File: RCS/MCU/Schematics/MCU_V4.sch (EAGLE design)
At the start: 28 parts, among them IC1 FT232RL, J1 MOTOR, J2 POWER, J3 SENSORS, Q2 8 MHz, U1 ATMEGA328P_TQFP

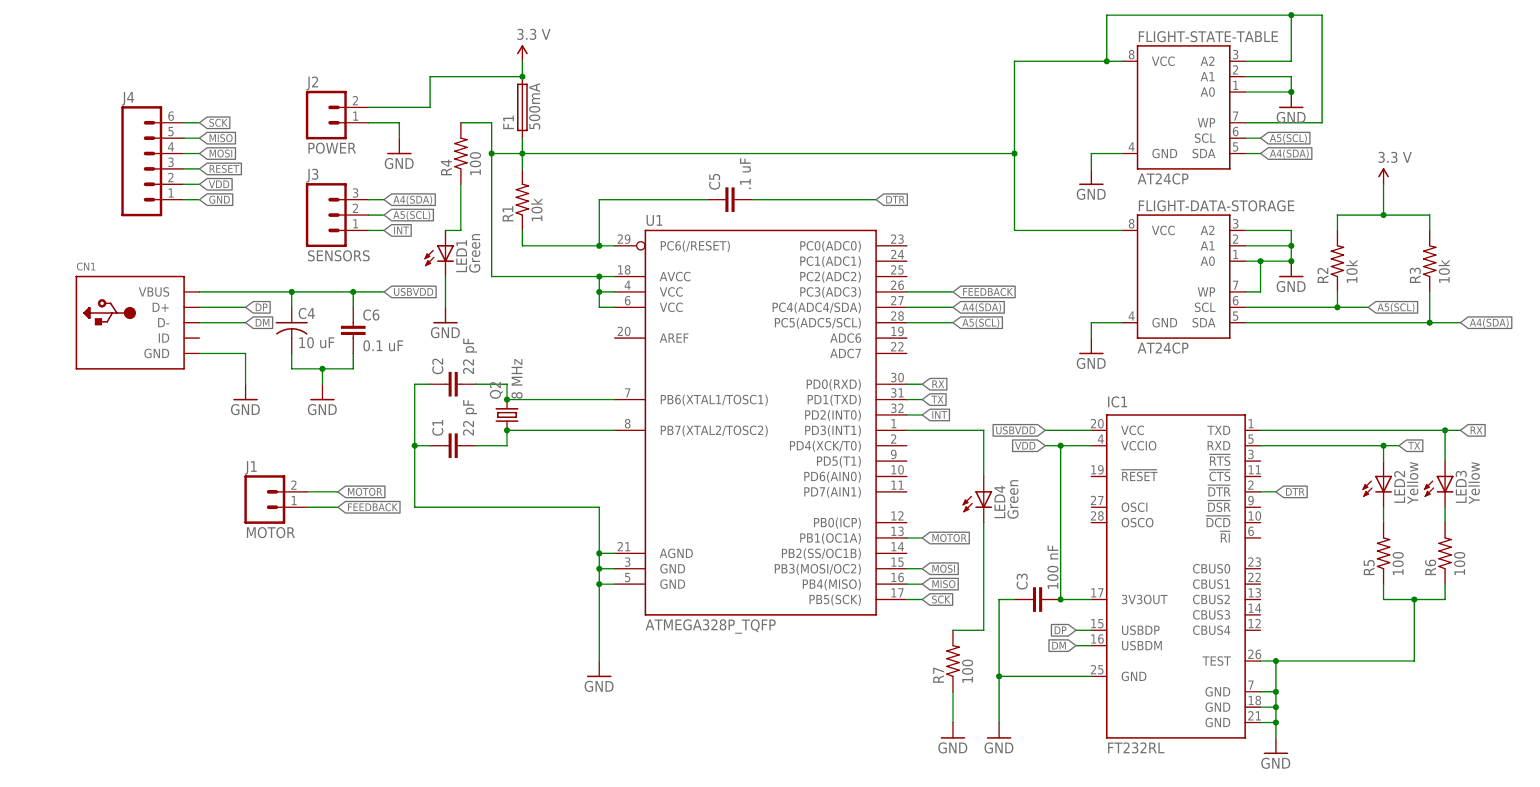
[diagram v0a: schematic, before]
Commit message: Updated INTEV Schematic
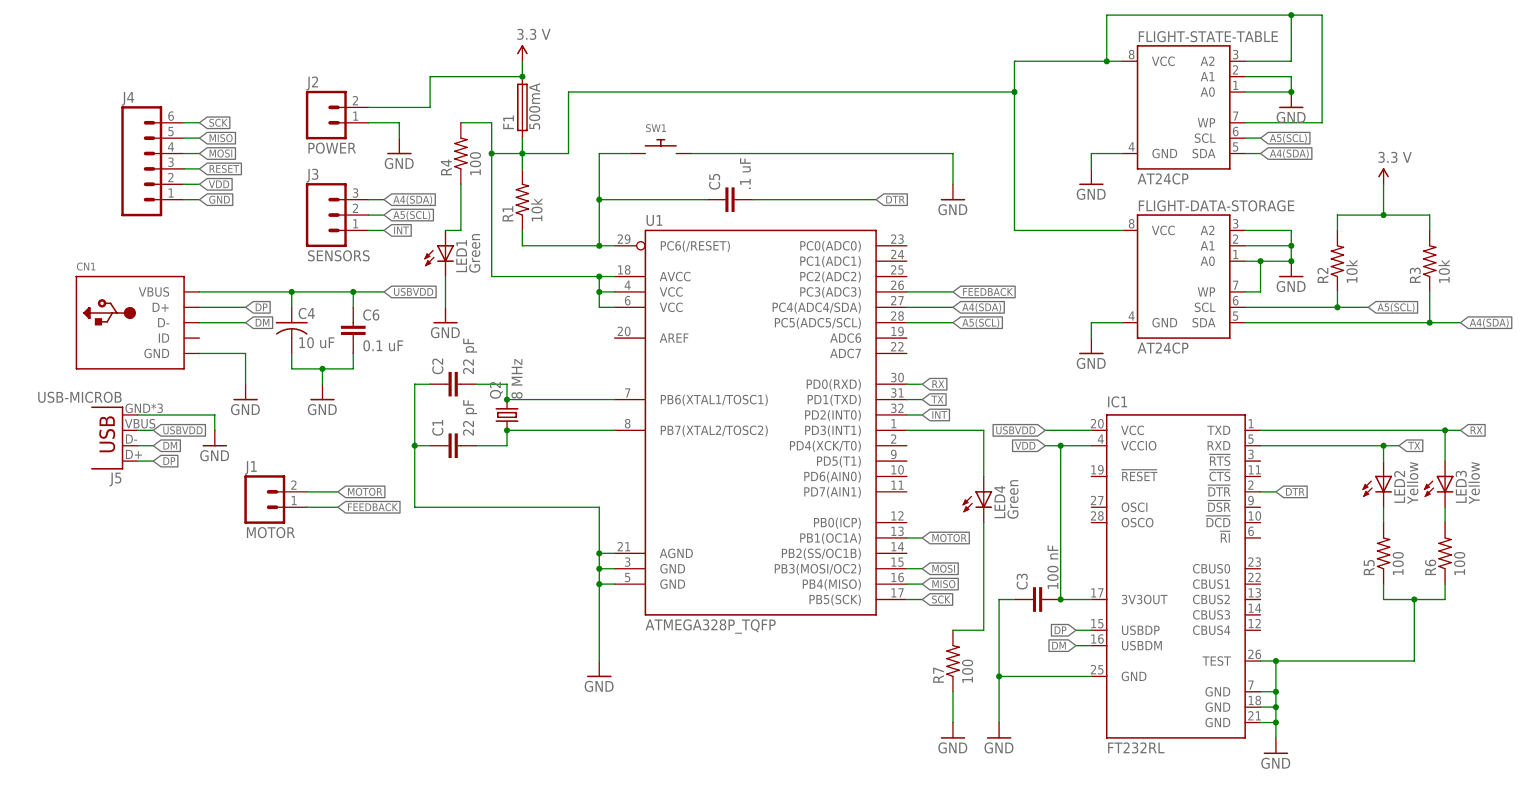
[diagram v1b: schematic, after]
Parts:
- added J5: USB-MICROB, SparkFun-Connectors:USB-MICROB
- added SW1: (no value), adafruit:SWITCH_PUSHBUTTONSOFTTOUCHSMD_SJ
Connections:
- net DM: now also J5.D-
- net DP: now also J5.D+
- net GND: now also J5.GND, SW1.P$2
- net RESET: now also SW1.P$1
- net USBVDD: now also J5.VBUS
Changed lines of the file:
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@@
 <part name="J3" library="SparkFun-Connectors" deviceset="M03" device="LOCK" value="SENSORS"/>
 <part name="J4" library="SparkFun-Connectors" deviceset="M06" device="LOCK"/>
+<part name="SW1" library="adafruit" deviceset="SWITCH_PUSHBUTTON" device="SOFTTOUCHSMD_SJ"/>
+<part name="GND13" library="supply1" deviceset="GND" device=""/>
+<part name="J5" library="SparkFun-Connectors" deviceset="USB" device="-MICROB"/>
+<part name="GND14" library="supply1" deviceset="GND" device=""/>
 </parts>
 <sheets>
@@
 <instance part="J3" gate="J$1" x="-12.7" y="78.74"/>
 <instance part="J4" gate="G$1" x="-40.64" y="86.36"/>
+<instance part="SW1" gate="G$1" x="43.18" y="88.9"/>
+<instance part="GND13" gate="1" x="91.44" y="81.28"/>
+<instance part="J5" gate="G$1" x="-45.72" y="45.72" rot="R180"/>
+<instance part="GND14" gate="1" x="-30.48" y="40.64"/>
 </instances>
 <busses>
@@
 <label x="-33.02" y="81.28" size="1.27" layer="95" xref="yes"/>
 </segment>
+<segment>
+<pinref part="GND13" gate="1" pin="GND"/>
+<wire x1="48.26" y1="88.9" x2="91.44" y2="88.9" width="0.1524" layer="91"/>
+<wire x1="91.44" y1="88.9" x2="91.44" y2="83.82" width="0.1524" layer="91"/>
+<pinref part="SW1" gate="G$1" pin="P$2"/>
+</segment>
+<segment>
+<pinref part="J5" gate="G$1" pin="GND"/>
+<wire x1="-43.18" y1="45.72" x2="-30.48" y2="45.72" width="0.1524" layer="91"/>
+<wire x1="-30.48" y1="45.72" x2="-30.48" y2="43.18" width="0.1524" layer="91"/>
+<pinref part="GND14" gate="1" pin="GND"/>
+</segment>
 </net>
 <net name="VDD" class="0">
@@
 <label x="111.76" y="7.62" size="1.27" layer="95" rot="R180" xref="yes"/>
 </segment>
+<segment>
+<pinref part="J5" gate="G$1" pin="D-"/>
+<wire x1="-43.18" y1="40.64" x2="-40.64" y2="40.64" width="0.1524" layer="91"/>
+<label x="-40.64" y="40.64" size="1.27" layer="95" xref="yes"/>
+</segment>
 </net>
 <net name="DP" class="0">
@@
 <wire x1="114.3" y1="10.16" x2="111.76" y2="10.16" width="0.1524" layer="91"/>
 <label x="111.76" y="10.16" size="1.27" layer="95" rot="R180" xref="yes"/>
+</segment>
+<segment>
+<pinref part="J5" gate="G$1" pin="D+"/>
+<wire x1="-43.18" y1="38.1" x2="-40.64" y2="38.1" width="0.1524" layer="91"/>
+<label x="-40.64" y="38.1" size="1.27" layer="95" xref="yes"/>
 </segment>
 </net>
@@
 <label x="-2.54" y="76.2" size="1.27" layer="95" xref="yes"/>
 <pinref part="J3" gate="J$1" pin="1"/>
-</segment>
-</net>
-<net name="N$5" class="0">
-<segment>
-<pinref part="FLIGHT-STATE-TABLE" gate="G$1" pin="A2"/>
-<wire x1="147.32" y1="104.14" x2="139.7" y2="104.14" width="0.1524" layer="91"/>
-<wire x1="147.32" y1="104.14" x2="147.32" y2="111.76" width="0.1524" layer="91"/>
-<pinref part="FLIGHT-STATE-TABLE" gate="G$1" pin="WP"/>
-<wire x1="139.7" y1="93.98" x2="152.4" y2="93.98" width="0.1524" layer="91"/>
-<wire x1="152.4" y1="93.98" x2="152.4" y2="111.76" width="0.1524" layer="91"/>
-<wire x1="152.4" y1="111.76" x2="147.32" y2="111.76" width="0.1524" layer="91"/>
-<pinref part="R1" gate="G$1" pin="2"/>
-<wire x1="147.32" y1="111.76" x2="116.84" y2="111.76" width="0.1524" layer="91"/>
-<wire x1="20.32" y1="86.36" x2="20.32" y2="88.9" width="0.1524" layer="91"/>
-<wire x1="20.32" y1="88.9" x2="20.32" y2="91.44" width="0.1524" layer="91"/>
-<wire x1="20.32" y1="88.9" x2="101.6" y2="88.9" width="0.1524" layer="91"/>
-<wire x1="101.6" y1="88.9" x2="101.6" y2="104.14" width="0.1524" layer="91"/>
-<junction x="20.32" y="88.9"/>
-<pinref part="FLIGHT-STATE-TABLE" gate="G$1" pin="VCC"/>
-<wire x1="101.6" y1="104.14" x2="116.84" y2="104.14" width="0.1524" layer="91"/>
-<pinref part="FLIGHT-DATA-STORAGE" gate="G$1" pin="VCC"/>
-<wire x1="116.84" y1="104.14" x2="119.38" y2="104.14" width="0.1524" layer="91"/>
-<wire x1="119.38" y1="76.2" x2="101.6" y2="76.2" width="0.1524" layer="91"/>
-<wire x1="101.6" y1="76.2" x2="101.6" y2="88.9" width="0.1524" layer="91"/>
-<junction x="101.6" y="88.9"/>
-<wire x1="116.84" y1="111.76" x2="116.84" y2="104.14" width="0.1524" layer="91"/>
-<junction x="116.84" y="104.14"/>
-<junction x="147.32" y="111.76"/>
-<pinref part="R4" gate="G$1" pin="2"/>
-<wire x1="10.16" y1="93.98" x2="15.24" y2="93.98" width="0.1524" layer="91"/>
-<wire x1="15.24" y1="93.98" x2="15.24" y2="88.9" width="0.1524" layer="91"/>
-<wire x1="15.24" y1="88.9" x2="20.32" y2="88.9" width="0.1524" layer="91"/>
-<wire x1="15.24" y1="88.9" x2="15.24" y2="68.58" width="0.1524" layer="91"/>
-<junction x="15.24" y="88.9"/>
-<pinref part="U1" gate="U$1" pin="VCC@6"/>
-<pinref part="U1" gate="U$1" pin="VCC@4"/>
-<pinref part="U1" gate="U$1" pin="AVCC"/>
-<wire x1="35.56" y1="68.58" x2="33.02" y2="68.58" width="0.1524" layer="91"/>
-<wire x1="33.02" y1="68.58" x2="33.02" y2="66.04" width="0.1524" layer="91"/>
-<wire x1="33.02" y1="66.04" x2="35.56" y2="66.04" width="0.1524" layer="91"/>
-<junction x="33.02" y="66.04"/>
-<wire x1="33.02" y1="66.04" x2="33.02" y2="63.5" width="0.1524" layer="91"/>
-<wire x1="33.02" y1="63.5" x2="35.56" y2="63.5" width="0.1524" layer="91"/>
-<wire x1="15.24" y1="68.58" x2="33.02" y2="68.58" width="0.1524" layer="91"/>
-<junction x="33.02" y="68.58"/>
-<pinref part="F1" gate="1" pin="1"/>
 </segment>
 </net>
@@
 <label x="106.68" y="43.18" size="1.27" layer="95" rot="R180" xref="yes"/>
 </segment>
+<segment>
+<pinref part="J5" gate="G$1" pin="VBUS"/>
+<wire x1="-43.18" y1="43.18" x2="-40.64" y2="43.18" width="0.1524" layer="91"/>
+<label x="-40.64" y="43.18" size="1.27" layer="95" xref="yes"/>
+</segment>
 </net>
 <net name="N$9" class="0">
@@
 <wire x1="33.02" y1="81.28" x2="50.8" y2="81.28" width="0.1524" layer="91"/>
 <junction x="33.02" y="73.66"/>
+<wire x1="33.02" y1="81.28" x2="33.02" y2="88.9" width="0.1524" layer="91"/>
+<junction x="33.02" y="81.28"/>
+<pinref part="SW1" gate="G$1" pin="P$1"/>
+<wire x1="33.02" y1="88.9" x2="38.1" y2="88.9" width="0.1524" layer="91"/>
 </segment>
 </net>
@@
 </segment>
 </net>
+<net name="N$1" class="0">
+<segment>
+<pinref part="U1" gate="U$1" pin="VCC@6"/>
+<wire x1="33.02" y1="63.5" x2="35.56" y2="63.5" width="0.1524" layer="91"/>
+<pinref part="U1" gate="U$1" pin="VCC@4"/>
+<wire x1="33.02" y1="66.04" x2="35.56" y2="66.04" width="0.1524" layer="91"/>
+<junction x="33.02" y="66.04"/>
+<wire x1="33.02" y1="66.04" x2="33.02" y2="63.5" width="0.1524" layer="91"/>
+<pinref part="U1" gate="U$1" pin="AVCC"/>
+<wire x1="35.56" y1="68.58" x2="33.02" y2="68.58" width="0.1524" layer="91"/>
+<wire x1="33.02" y1="68.58" x2="33.02" y2="66.04" width="0.1524" layer="91"/>
+<junction x="33.02" y="68.58"/>
+<pinref part="F1" gate="1" pin="1"/>
+<pinref part="R1" gate="G$1" pin="2"/>
+<wire x1="20.32" y1="86.36" x2="20.32" y2="88.9" width="0.1524" layer="91"/>
+<wire x1="20.32" y1="88.9" x2="20.32" y2="91.44" width="0.1524" layer="91"/>
+<junction x="20.32" y="88.9"/>
+<pinref part="R4" gate="G$1" pin="2"/>
+<wire x1="10.16" y1="93.98" x2="15.24" y2="93.98" width="0.1524" layer="91"/>
+<wire x1="15.24" y1="93.98" x2="15.24" y2="88.9" width="0.1524" layer="91"/>
+<wire x1="15.24" y1="88.9" x2="20.32" y2="88.9" width="0.1524" layer="91"/>
+<junction x="15.24" y="88.9"/>
+<wire x1="15.24" y1="88.9" x2="15.24" y2="68.58" width="0.1524" layer="91"/>
+<wire x1="15.24" y1="68.58" x2="33.02" y2="68.58" width="0.1524" layer="91"/>
+<wire x1="20.32" y1="88.9" x2="27.94" y2="88.9" width="0.1524" layer="91"/>
+<wire x1="27.94" y1="88.9" x2="27.94" y2="99.06" width="0.1524" layer="91"/>
+<pinref part="FLIGHT-STATE-TABLE" gate="G$1" pin="A2"/>
+<wire x1="147.32" y1="104.14" x2="139.7" y2="104.14" width="0.1524" layer="91"/>
+<wire x1="147.32" y1="104.14" x2="147.32" y2="111.76" width="0.1524" layer="91"/>
+<pinref part="FLIGHT-STATE-TABLE" gate="G$1" pin="WP"/>
+<wire x1="139.7" y1="93.98" x2="152.4" y2="93.98" width="0.1524" layer="91"/>
+<wire x1="152.4" y1="93.98" x2="152.4" y2="111.76" width="0.1524" layer="91"/>
+<wire x1="152.4" y1="111.76" x2="147.32" y2="111.76" width="0.1524" layer="91"/>
+<wire x1="147.32" y1="111.76" x2="116.84" y2="111.76" width="0.1524" layer="91"/>
+<wire x1="101.6" y1="76.2" x2="101.6" y2="99.06" width="0.1524" layer="91"/>
+<pinref part="FLIGHT-STATE-TABLE" gate="G$1" pin="VCC"/>
+<wire x1="101.6" y1="99.06" x2="101.6" y2="104.14" width="0.1524" layer="91"/>
+<wire x1="101.6" y1="104.14" x2="116.84" y2="104.14" width="0.1524" layer="91"/>
+<pinref part="FLIGHT-DATA-STORAGE" gate="G$1" pin="VCC"/>
+<wire x1="116.84" y1="104.14" x2="119.38" y2="104.14" width="0.1524" layer="91"/>
+<wire x1="119.38" y1="76.2" x2="101.6" y2="76.2" width="0.1524" layer="91"/>
+<wire x1="116.84" y1="111.76" x2="116.84" y2="104.14" width="0.1524" layer="91"/>
+<junction x="116.84" y="104.14"/>
+<junction x="147.32" y="111.76"/>
+<wire x1="27.94" y1="99.06" x2="101.6" y2="99.06" width="0.1524" layer="91"/>
+<junction x="101.6" y="99.06"/>
+</segment>
+</net>
